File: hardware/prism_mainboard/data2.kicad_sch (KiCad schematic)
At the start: 2 parts, among them IC3 USB3320C-EZK, J1 503398-1892

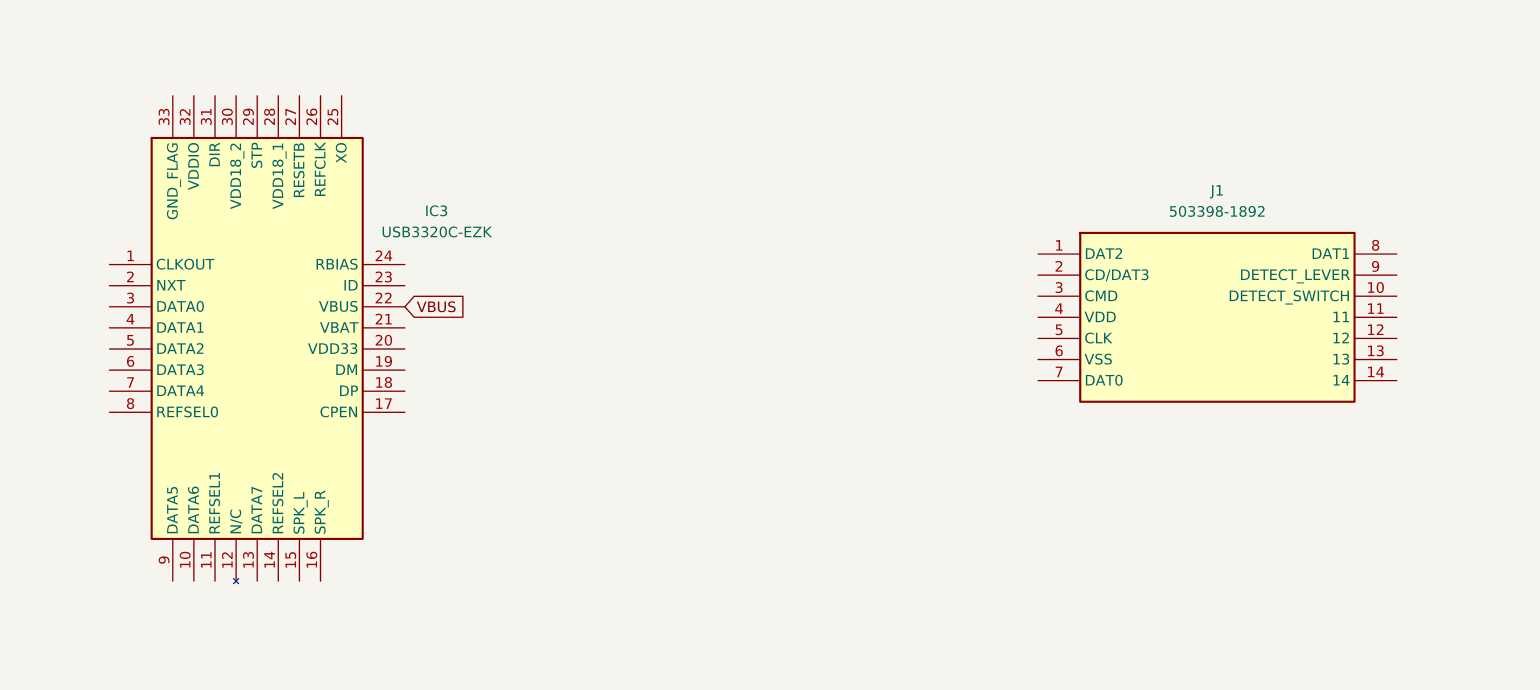
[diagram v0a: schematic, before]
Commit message: Updates
Mostly Schematic updates, nothing too big. Added a few datasheets
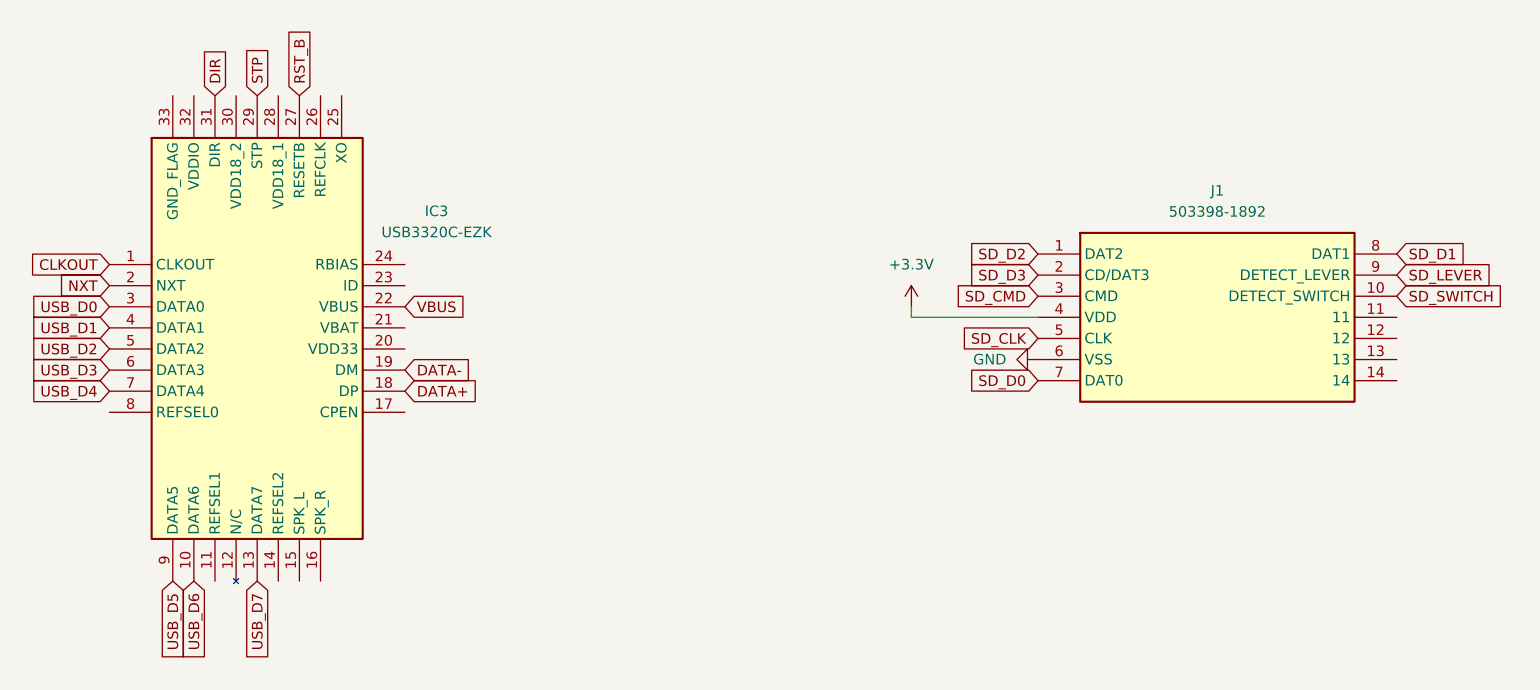
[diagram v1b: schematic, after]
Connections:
- net CLKOUT: now reaches IC3.1 (CLKOUT)
- net USB_D6: now reaches IC3.10 (DATA6)
- net USB_D7: now reaches IC3.13 (DATA7)
- net DATA+: now reaches IC3.18 (DP)
- net DATA-: now reaches IC3.19 (DM)
- net NXT: now reaches IC3.2 (NXT)
- net RST_B: now reaches IC3.27 (RESETB)
- net STP: now reaches IC3.29 (STP)
- net USB_D0: now reaches IC3.3 (DATA0)
- net DIR: now reaches IC3.31 (DIR)
- net USB_D1: now reaches IC3.4 (DATA1)
- net USB_D2: now reaches IC3.5 (DATA2)
- net USB_D3: now reaches IC3.6 (DATA3)
- net USB_D4: now reaches IC3.7 (DATA4)
- net USB_D5: now reaches IC3.9 (DATA5)
- net SD_D2: now reaches J1.1 (DAT2)
- net SD_SWITCH: now reaches J1.10 (DETECT_SWITCH)
- net SD_D3: now reaches J1.2 (CD/DAT3)
- net SD_CMD: now reaches J1.3 (CMD)
- net +3.3V: now reaches J1.4 (VDD)
- net SD_CLK: now reaches J1.5 (CLK)
- net GND: now reaches J1.6 (VSS)
- net SD_D0: now reaches J1.7 (DAT0)
- net SD_D1: now reaches J1.8 (DAT1)
- net SD_LEVER: now reaches J1.9 (DETECT_LEVER)
